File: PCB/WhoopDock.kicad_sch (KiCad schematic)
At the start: 45 parts, among them J1 BetaFPV_BT2.0, J2 BetaFPV_BT2.0, J3 BetaFPV_BT2.0, J4 BetaFPV_BT2.0, J5 BetaFPV_BT2.0, J6 BetaFPV_BT2.0, SW1 SW_Push, U1 ESP32-S3-WROOM-1, U10 BQ25890RTWR, U2 CH224K, U3 XL1509-5.0E1, U4 BQ25890RTWR, U5 RT9193-33GB, U6 BQ25890RTWR, U7 BQ25890RTWR, U8 BQ25890RTWR, U9 BQ25890RTWR

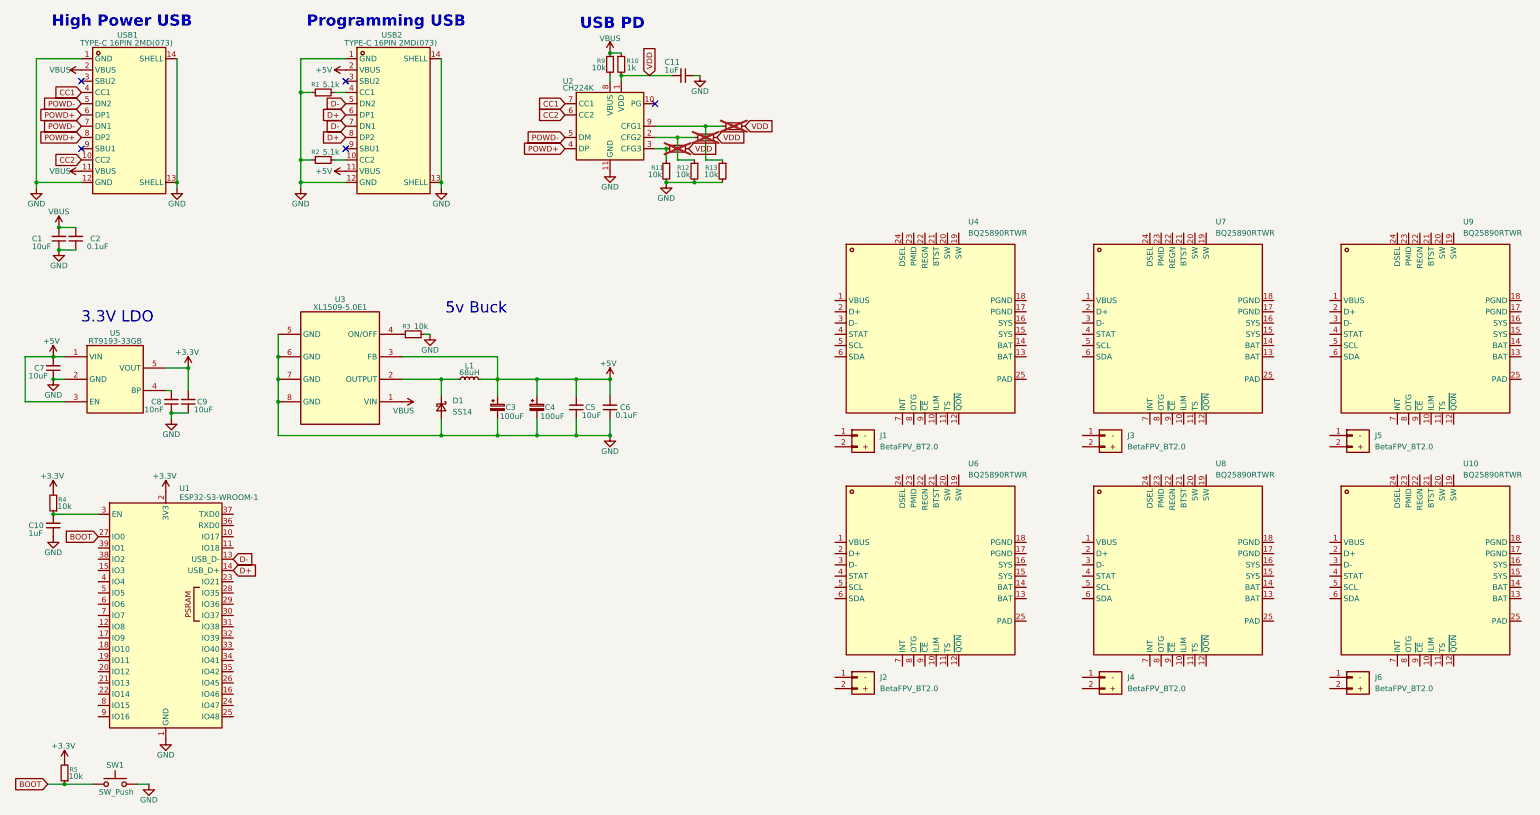
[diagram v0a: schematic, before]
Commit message: checkpoint
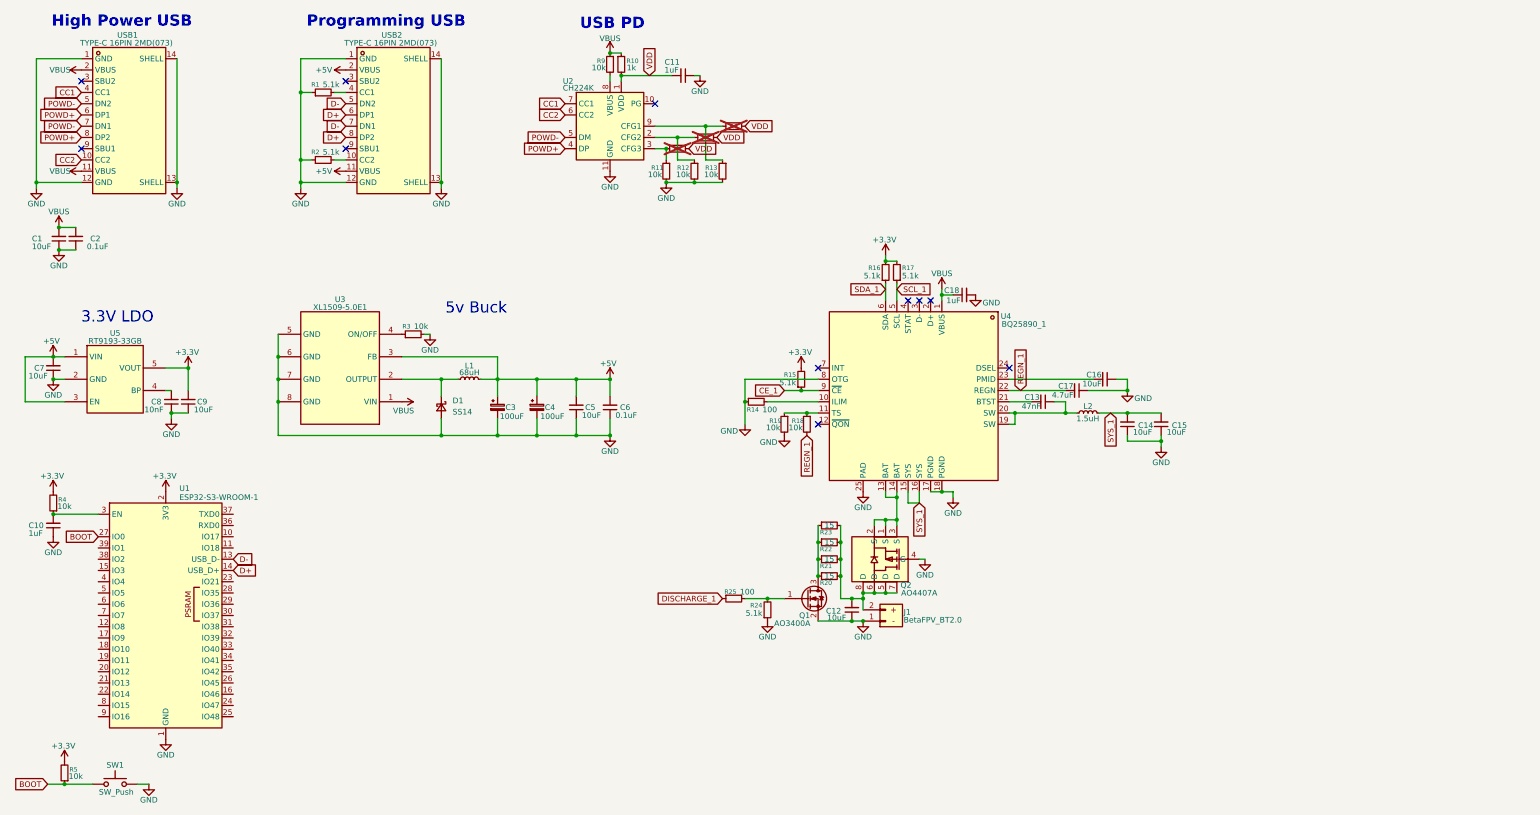
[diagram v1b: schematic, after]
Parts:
- removed J2, J3, J4, J5, J6: BetaFPV_BT2.0, easyeda2kicad:BetaFPV BT2.0, symbol WhoopDock:BetaFPV_BT2.0
- removed U10, U6, U7, U8, U9: BQ25890RTWR, easyeda2kicad:WQFN-24_L4.0-W4.0-P0.50-BL-EP, symbol WhoopDock:BQ25890RTWR
- added C12, C14, C15, C16: 10uF, Capacitor_SMD:C_0805_2012Metric, symbol Device:C_Small
- added C13: 47nF, Capacitor_SMD:C_0603_1608Metric, symbol Device:C_Small
- added C17: 4.7uF, Capacitor_SMD:C_0603_1608Metric, symbol Device:C_Small
- added C18: 1uF, Capacitor_SMD:C_0603_1608Metric, symbol Device:C_Small
- added L2: 1.5uH, Inductor_SMD:L_APV_APH0420, symbol Device:L_Small
- added Q1: AO3400A, Package_TO_SOT_SMD:SOT-23, symbol Transistor_FET:AO3400A
- added Q2: AO4407A, easyeda2kicad:SOIC-8_L4.9-W3.9-P1.27-LS6.0-BL, symbol WhoopDock:AO4407A
- added R14, R25: 100, Resistor_SMD:R_0603_1608Metric, symbol Device:R_Small
- added R15, R16, R17, R24: 5.1k, Resistor_SMD:R_0603_1608Metric, symbol Device:R_Small
- added R18, R19: 10k, Resistor_SMD:R_0603_1608Metric, symbol Device:R_Small
- added R20, R21, R22, R23: 15, Resistor_SMD:R_2512_6332Metric, symbol Device:R_Small
- U4: value BQ25890RTWR -> BQ25890_1
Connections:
- net +3.3V: now also R15.2, R16.2, R17.2
- net GND: now also J1.1 (Pin_1), U4.17 (PGND), U4.18 (PGND), U4.25 (PAD), U4.8 (OTG), C12.1, C14.1, C15.1, C16.1, C17.1, C18.2, Q1.2 (S), Q2.4 (G), R14.1, R19.2, R24.1
- net VBUS: now also U4.1 (VBUS), C18.1
- net at J1.2 (Pin_2): now also C12.2, Q2.5 (D), Q2.6 (D), Q2.7 (D), Q2.8 (D), R20.2, R21.2, R22.2, R23.2
- net at U4.10 (ILIM): now also R14.2
- net at U4.11 (TS): now also R18.1, R19.1
- net at U4.13 (BAT): now also U4.14 (BAT), Q2.1 (S), Q2.2 (S), Q2.3 (S)
- net SYS_1: now reaches U4.15 (SYS)
- net SYS_1: now also U4.16 (SYS), C14.2, C15.2, L2.2
- net at U4.19 (SW): now also U4.20 (SW), C13.1, L2.1
- net at U4.21 (BTST): now also C13.2
- net REGN_1: now reaches U4.22 (REGN)
- net REGN_1: now also C17.2, R18.2
- net at U4.23 (PMID): now also C16.2
- net SCL_1: now reaches U4.5 (SCL)
- net SCL_1: now also R17.1
- net SDA_1: now reaches U4.6 (SDA)
- net SDA_1: now also R16.1
- net CE_1: now reaches U4.9 (~{CE})
- net CE_1: now also R15.1
- new net: Q1.1 (G), R24.2, R25.2
- new net: Q1.3 (D), R20.1, R21.1, R22.1, R23.1
- new net DISCHARGE_1: R25.1
- no-connect marks 5 -> 11
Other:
- moved on the sheet: J1, U4
